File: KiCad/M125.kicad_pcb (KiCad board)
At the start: 2 copper layers, 13.2 x 13.5 mm, 9 parts, among them J1 Shelly, U1 ESP32-PICO-MINI-02

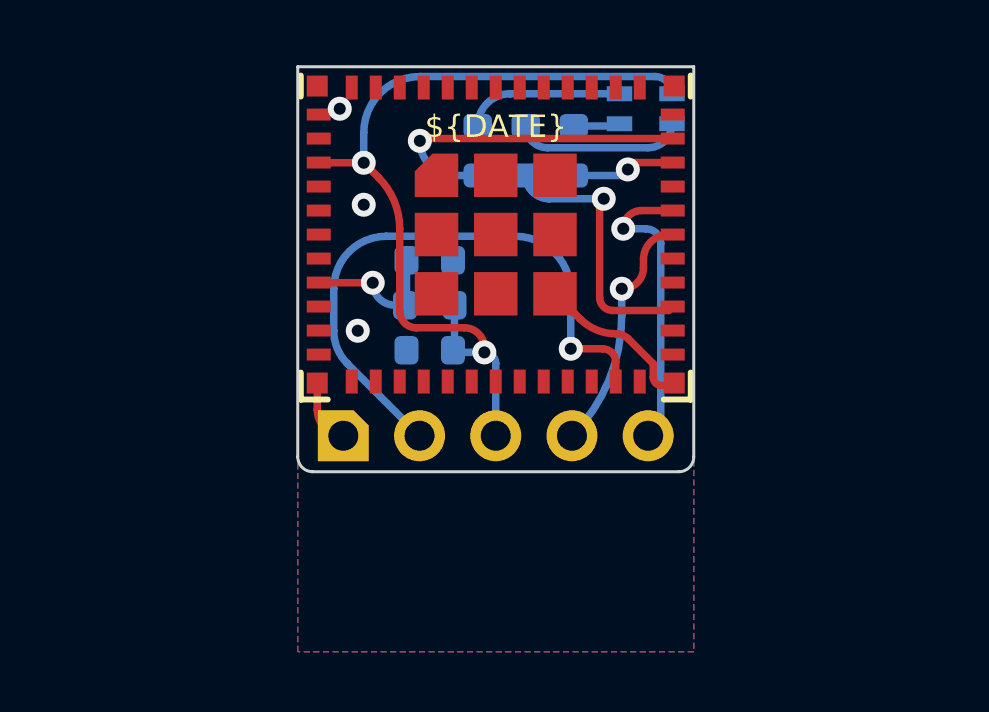
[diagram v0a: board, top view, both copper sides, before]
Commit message: Tweak PCBs
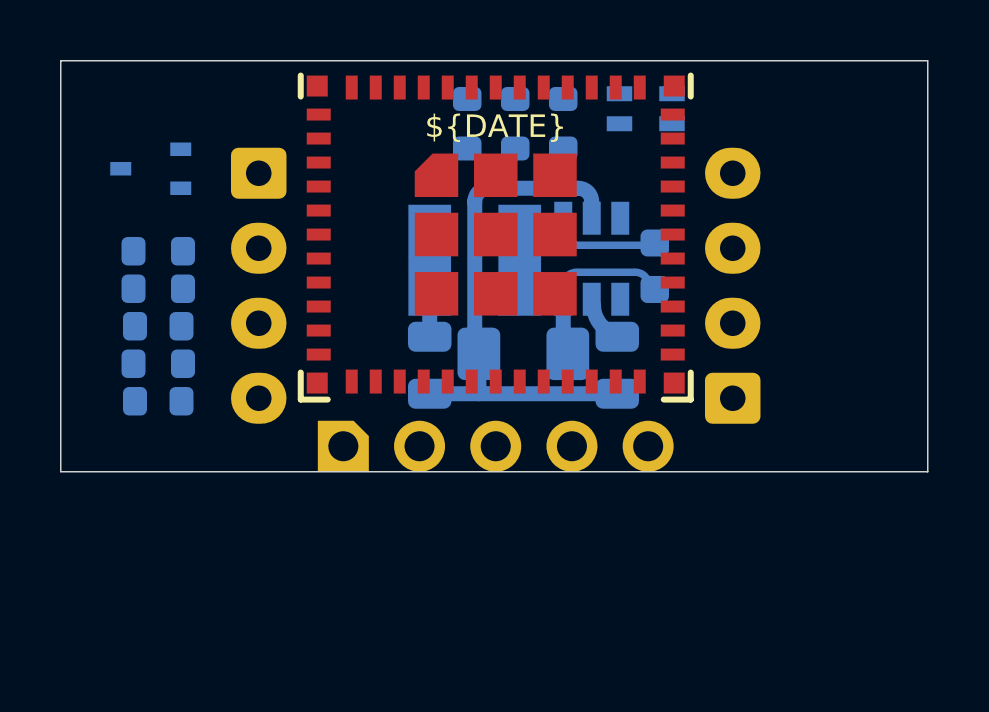
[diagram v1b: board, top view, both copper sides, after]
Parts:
- added C3: 0.1uF, RevK:Hidden, F.Cu at (74.9, 55.4)
- added C4: 2.2uF, RevK:Hidden, F.Cu at (91.3, 37.4)
- added C5: 10uF, RevK:Hidden, F.Cu at (93.4, 37.4)
- added D2: Schottky, RevK:Hidden, F.Cu at (72.8, 55.4)
- added J1: Conn_01x04, RevK:Molex_MiniSPOX_H4RA, F.Cu at (92.1, 45.9)
- added J2: Conn_01x04, RevK:Molex_MiniSPOX_H4RA, F.Cu at (107.9, 45.9)
- added L1: 6.8uH, RevK:Hidden, F.Cu at (81.2, 50.1)
- added Q1: PMF250XNEX, Package_TO_SOT_SMD:SOT-323_SC-70, B.Cu at (88.5, 42.0)
- added R5: 100k 1% or 0R, RevK:R_0603, B.Cu at (88.8, 46.0)
- added R6: 30k 1% or NF, RevK:R_0603, B.Cu at (88.8, 44.8)
- added U2: LMR16006+FB, RevK:RegulatorBlockFB, B.Cu at (103.2, 45.0)
- R4: footprint RevK:Pad_0603_Bridged -> RevK:R_0603
- moved C1 9.31 mm to (88.8, 47.2)
- moved R4 9.26 mm to (88.8, 48.5)
- moved C2 9.21 mm to (88.8, 49.8)
- moved R1 0.97 mm to (99.0, 40.5)
- moved R2 0.97 mm to (102.2, 40.5)
- moved R3 0.97 mm to (100.7, 40.5)
- moved J3 0.35 mm to (100.0, 51.2)
- renumbered J1 to J3
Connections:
- U1 pad 18: unconnected-(U1-Pad18) -> NFCTX
- U1 pad 20: unconnected-(U1-Pad20) -> NFCRX
- U1 pad 21: unconnected-(U1-Pad21) -> DATA
- U1 pad 28: unconnected-(U1-Pad28) -> SEND
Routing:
- net +3V3: track 28.6 -> 0.00 mm, vias 2 -> 0
- net GPIO0: track 20.1 -> 0.00 mm, vias 1 -> 0
- net R: track 11.0 -> 0.00 mm, vias 1 -> 0
- net TX: track 10.1 -> 0.00 mm, vias 1 -> 0
- net B: track 9.08 -> 0.00 mm, vias 1 -> 0
- net RX: track 8.10 -> 0.00 mm, vias 1 -> 0
- net GND: track 7.69 -> 0.00 mm, vias 3 -> 0
- net Net-(D1-Pad4): track 5.68 -> 0.00 mm
- net Net-(D1-Pad2): track 5.30 -> 0.00 mm
- net EN: track 4.80 -> 0.00 mm, vias 1 -> 0
- net G: track 3.48 -> 0.00 mm, vias 1 -> 0
- net Net-(D1-Pad3): track 1.56 -> 0.00 mm
- removed copper zone on B.Cu, net GND
- removed copper zone on F.Cu, net GND
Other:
- board size 13.2 x 13.5 mm -> 28.9 x 13.7 mm
- board text removed: "Generic0"
